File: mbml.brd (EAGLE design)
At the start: 89.7 x 57.1 mm, 30 parts, among them K1 G5SB, Q1 2N2222, U1 LINEAR_REG_5V, U2 PHOTOCOUPLER, X1 43160-1102, X10 CON-2B2B-XH-A(LF)(SN), X2 CON-2, X3 CON-2B2B-XH-A(LF)(SN), X4 CON-2B2B-XH-A(LF)(SN), X5 CON-2B2B-XH-A(LF)(SN), X6 CON-2B2B-XH-A(LF)(SN), X7 CON-2B2B-XH-A(LF)(SN), X8 CON-2B2B-XH-A(LF)(SN), X9 CON-2B2B-XH-A(LF)(SN)

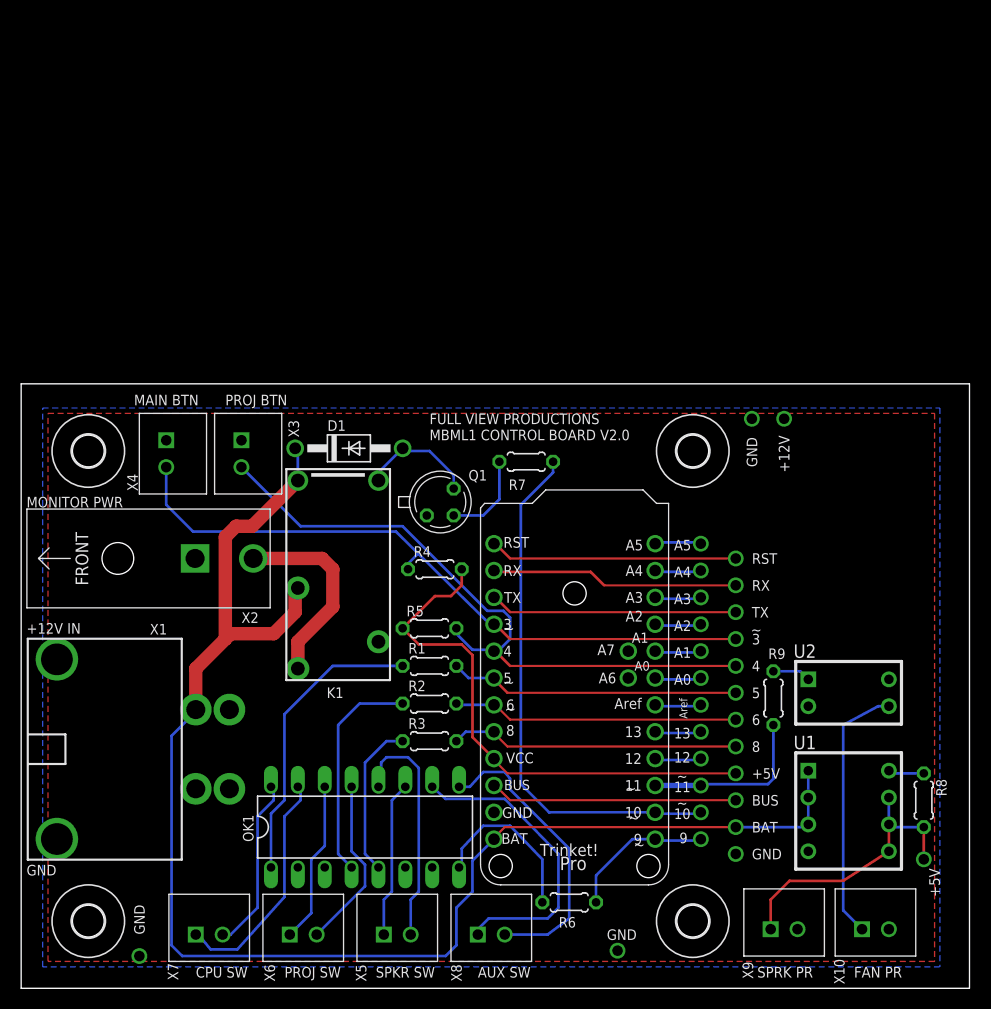
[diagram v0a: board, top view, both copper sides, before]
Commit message: Starting major overhaul
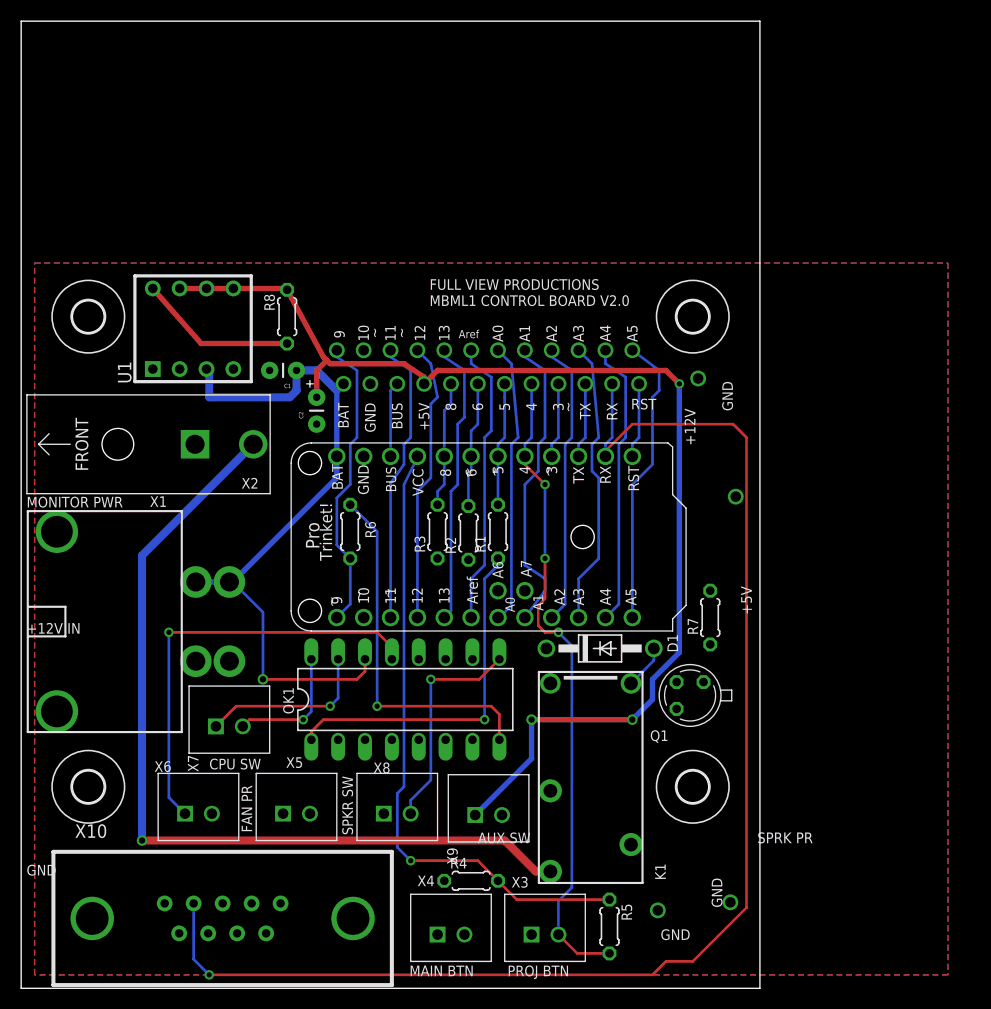
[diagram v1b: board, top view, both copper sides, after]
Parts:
- removed R9: 470, resistor:0204/5
- removed U2: PHOTOCOUPLER, TinkerTech:DIP-4
- added C1: (no value), SparkFun-Passives:CAP-PTH-SMALL
- added C2: (no value), TinkerTech:CAP-PTH-SMALL-POL
- R7: value 1.54k -> 1.5k
- X10: value CON-2B2B-XH-A(LF)(SN) -> CON_DB9VERT; device FVP:CON_2-2.5MM_TH -> TinkerTech:D09P24A4GV00LF
- moved U1 76.9 mm to (16.3, 62.4), turned to 0 degrees
- moved R8 75.6 mm to (25.1, 63.5), turned to 90 degrees
- moved X10 61.7 mm to (19.1, 6.60)
- moved X3 53.8 mm to (49.5, 5.08), turned to 0 degrees
- moved X4 52.8 mm to (40.6, 5.08), turned to 0 degrees
- moved R6 40.7 mm to (31.1, 43.2), turned to 270 degrees
- moved R5 32.9 mm to (55.6, 5.84), turned to 90 degrees
- moved K1 30.6 mm to (53.8, 21.2)
- moved D1 30.4 mm to (54.7, 32.1)
- moved X9 30.0 mm to (44.2, 16.4)
- moved Q1 29.9 mm to (63.2, 27.7), turned to 180 degrees
- moved R4 29.7 mm to (42.5, 10.2)
- moved R7 22.8 mm to (65.2, 35.1), turned to 270 degrees
- moved R3 19.8 mm to (39.4, 43.2), turned to 90 degrees
- moved X7 19.8 mm to (19.7, 24.8)
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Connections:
- net N$1 renamed D3
- net N$10 renamed D8
- net N$18 renamed D9
- net N$2 renamed D4
- net N$3 renamed TRANS_COLLECTOR
- net N$35 renamed D10
- net N$4 renamed D5
- net N$5 renamed TRANS_BASE
- net N$9 renamed D6
- removed net N$13: OK1.14, X6.P$1
- removed net N$46: R9.1, U2.1
- removed net N$47: R9.2, U$1.11
- removed net N$49: U2.3, X10.P$1
- new net A0: U$1.A0
- new net A1: U$1.A1
- new net A2: U$1.A2
- new net A3: U$1.A3
- new net A4: U$1.A4
- new net A5: U$1.A5
- new net A6: U$1.A6
- new net A7: U$1.A7
- new net AREF: U$1.AREF
- new net D11: U$1.11
- new net D12: U$1.12
- new net D13: U$1.13
- new net RST: U$1.RST
- new net RX: U$1.RX, X10.2
- new net TX: U$1.TX, X10.3
- net +12V: now also C1.1, OK1.14; no longer U2.4
- net +5V: now also C2.POS
- net GND: now also C1.2, C2.NEG, X10.5, X6.P$2; no longer U2.2, X10.P$2
- net N$14: now also X6.P$1; no longer X6.P$2
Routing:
- net RX: track 0.00 -> 127.8 mm, vias 0 -> 2
- net +5V: track 27.1 -> 111.6 mm, vias 1 -> 5
- net +12V: track 138.2 -> 65.9 mm
- net MON_PWR: track 18.7 -> 81.6 mm, vias 0 -> 1
- net D10: track 45.5 -> 0.00 mm, vias 0 -> 1
- net D3: track 41.1 -> 7.12 mm, vias 0 -> 1
- net MCU_VCC: track 27.1 -> 59.6 mm, vias 0 -> 1
- net A1: track 0.00 -> 28.7 mm, vias 0 -> 1
- net N$19: track 28.6 -> 0.00 mm
- net D11: track 0.00 -> 27.6 mm, vias 0 -> 1
- net A5: track 0.00 -> 27.6 mm, vias 0 -> 1
- net A3: track 0.00 -> 27.1 mm, vias 0 -> 1
- net A4: track 0.00 -> 27.1 mm, vias 0 -> 1
- net A2: track 0.00 -> 27.1 mm, vias 0 -> 1
- net AREF: track 0.00 -> 27.1 mm, vias 0 -> 1
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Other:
- board size 89.7 x 57.1 mm -> 69.8 x 91.4 mm
- board text removed: "PROJ SW"
